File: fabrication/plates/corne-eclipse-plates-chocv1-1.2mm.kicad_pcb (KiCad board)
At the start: 2 copper layers, 272.4 x 180.5 mm, 44 parts

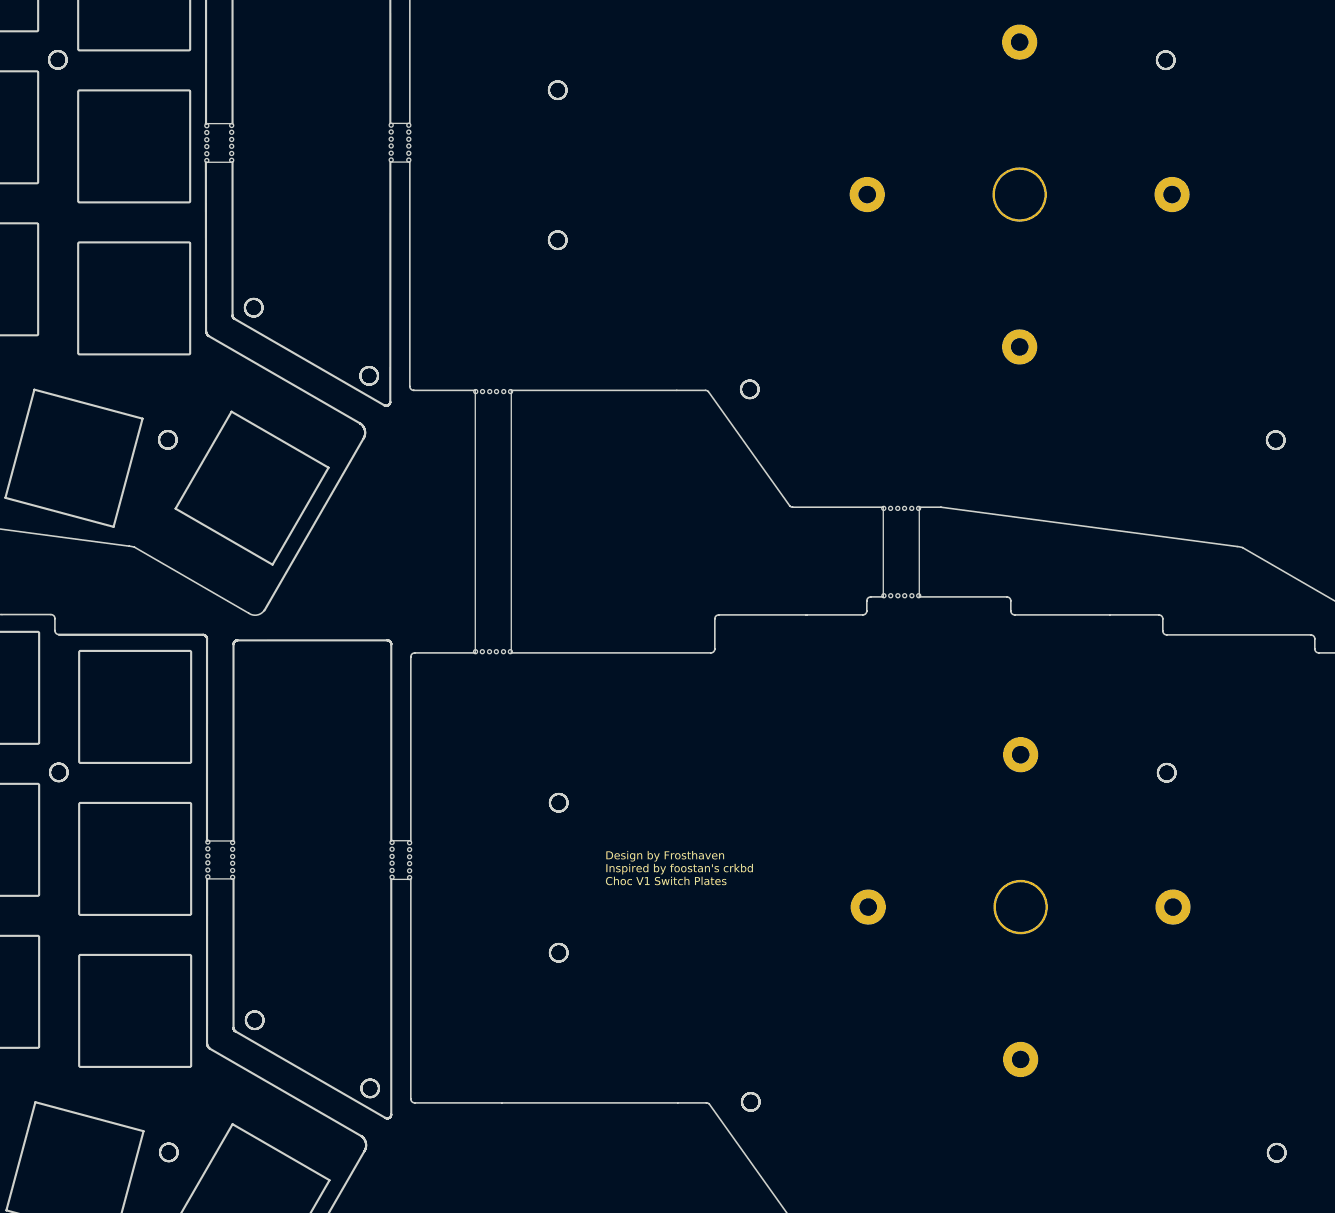
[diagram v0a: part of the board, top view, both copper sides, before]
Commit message: wip
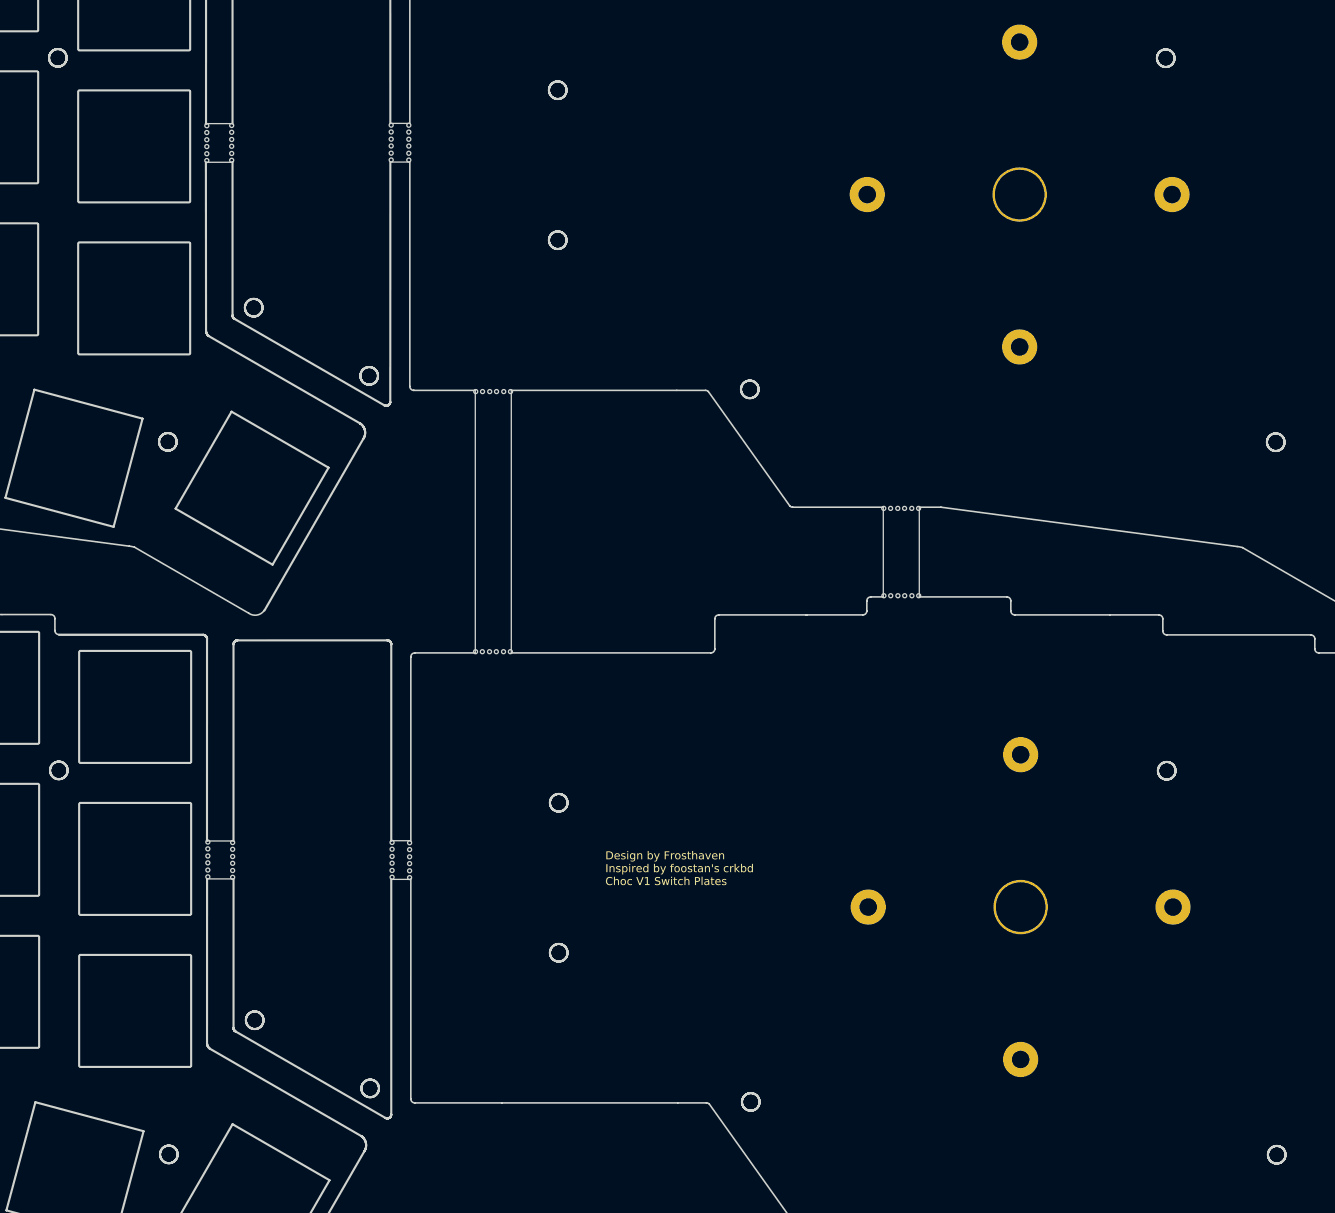
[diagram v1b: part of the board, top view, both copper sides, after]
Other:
- outline, holes or cut-outs redrawn
